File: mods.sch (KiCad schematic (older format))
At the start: 22 parts

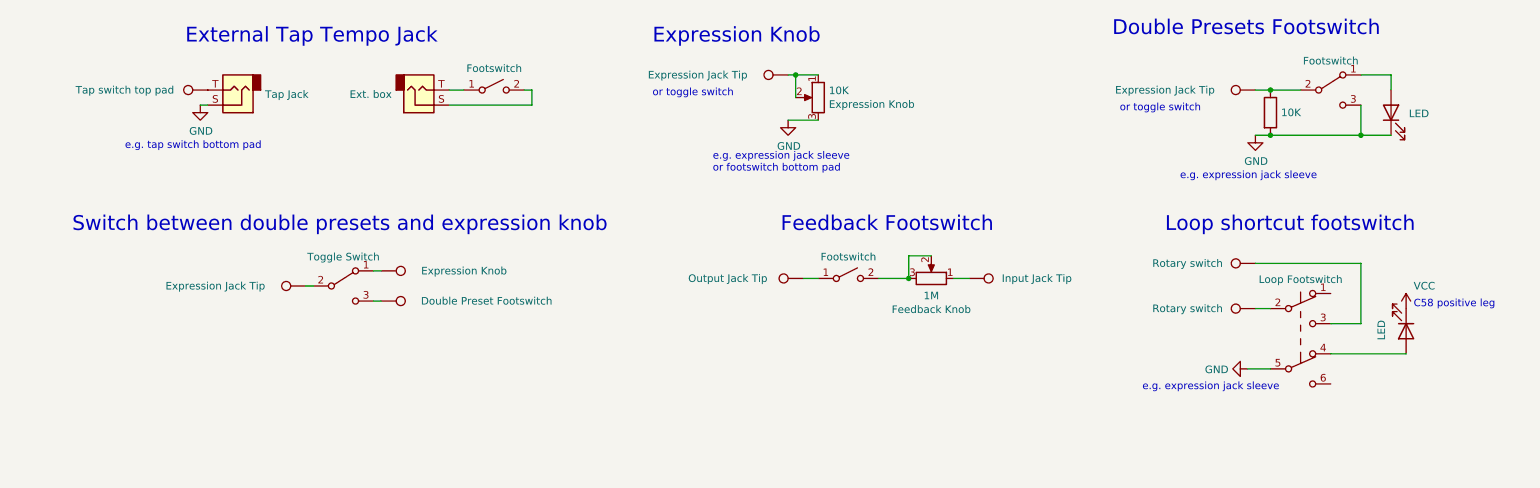
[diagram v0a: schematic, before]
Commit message: readyish
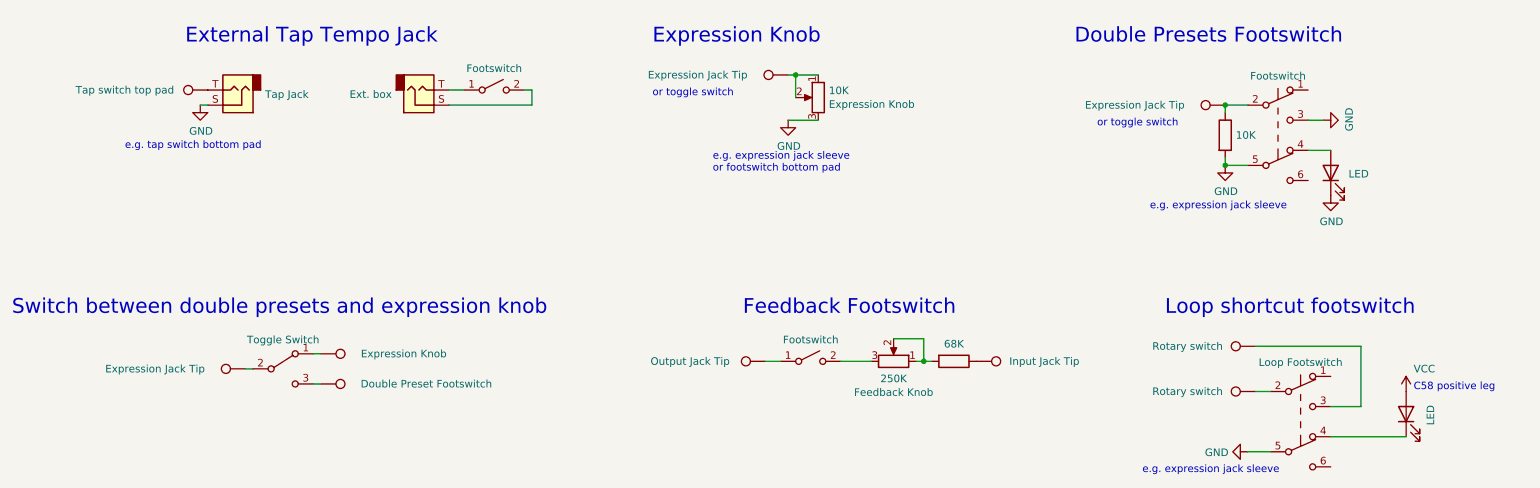
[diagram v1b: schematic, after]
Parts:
- removed D?: LED, symbol Device:LED
- removed R?: 10K, symbol Device:R
- removed SW?: Footswitch, symbol Switch:SW_SPDT
- removed TP?: Expression Jack Tip, symbol Connector:TestPoint
- added D?: LED, symbol Device:LED
- added R?: 10K, symbol Device:R
- added R?: 68K, symbol Device:R
- added SW?: Footswitch, symbol Switch:SW_Push_DPDT
- added TP?: Expression Jack Tip, symbol Connector:TestPoint
- renumbered 1M to 250K
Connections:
- net GND: now also D?.1 (K), R?.2, SW?.3 (C), SW?.5 (B)
- net VCC: now also D?.2 (A); no longer D?.1 (K)
- net at 250K.3, SW?.2 (B): no longer 250K.2
- net at TP?.1: now also R?.1; no longer 250K.1
- net at SW?.4 (A): now also D?.1 (K); no longer D?.2 (A)
- new net: 250K.1, 250K.2, R?.2
- new net: R?.1, SW?.2 (B), TP?.1
- new net: D?.2 (A), SW?.4 (A)
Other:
- moved on the sheet: 250K
